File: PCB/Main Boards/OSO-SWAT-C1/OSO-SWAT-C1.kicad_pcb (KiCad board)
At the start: 4 copper layers, 24.4 x 24.4 mm, 36 parts, among them J1 OSO_SWD, J2 FH19C-9S-0.5SH_10_, Q1 Q_Photo_NPN, Q2 Q_NMOS_GSD, U1 ATSAML22J18A-MUT, U2 MIC5365-3.3YC5-TR, X1 Crystal

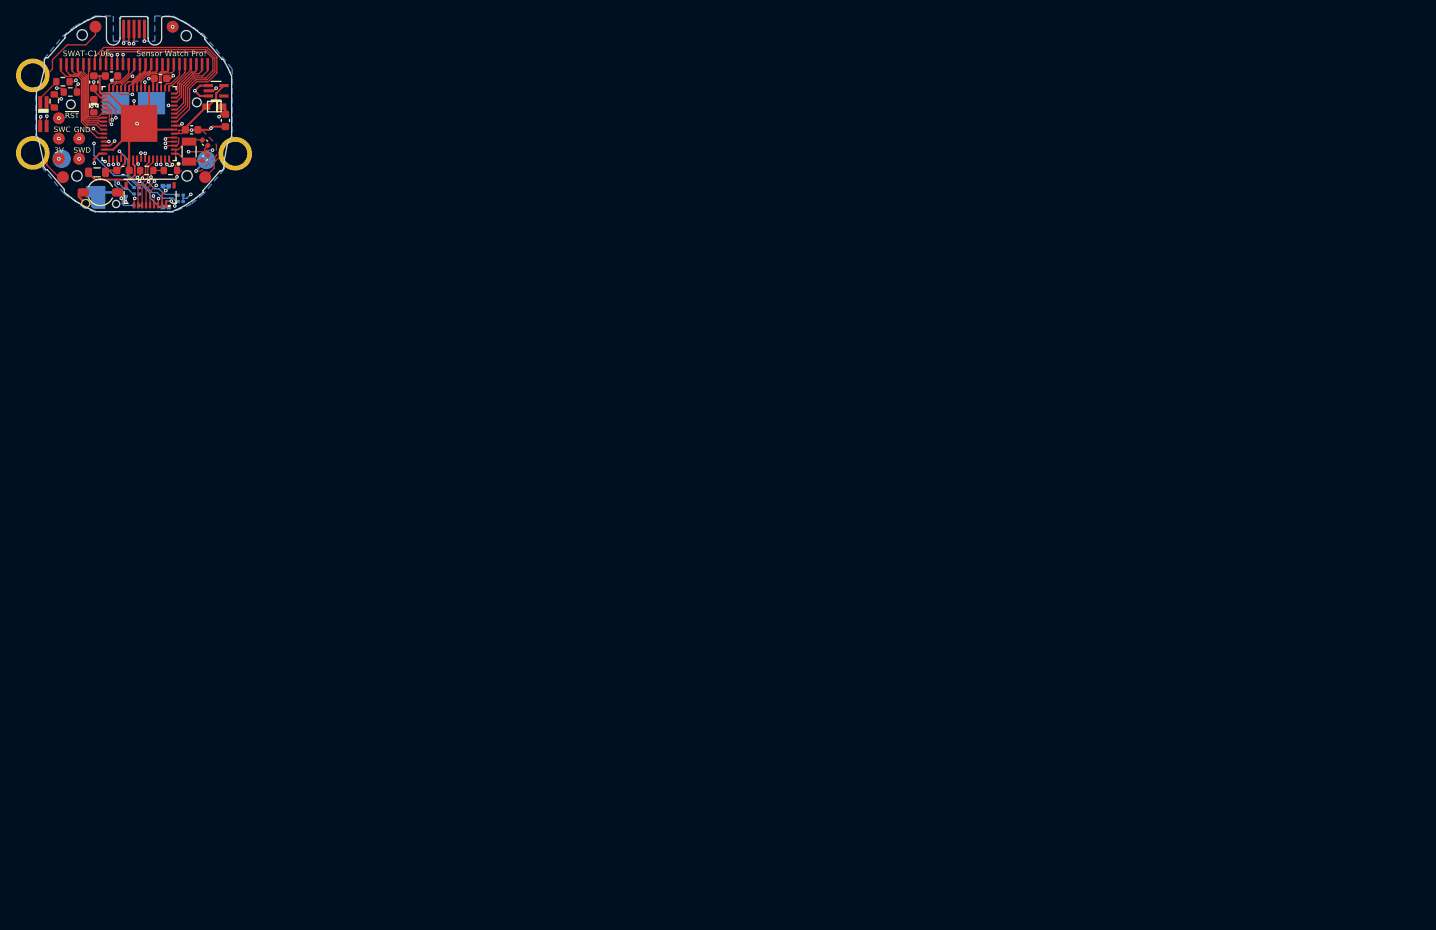
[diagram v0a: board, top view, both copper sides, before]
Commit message: Initial commit.
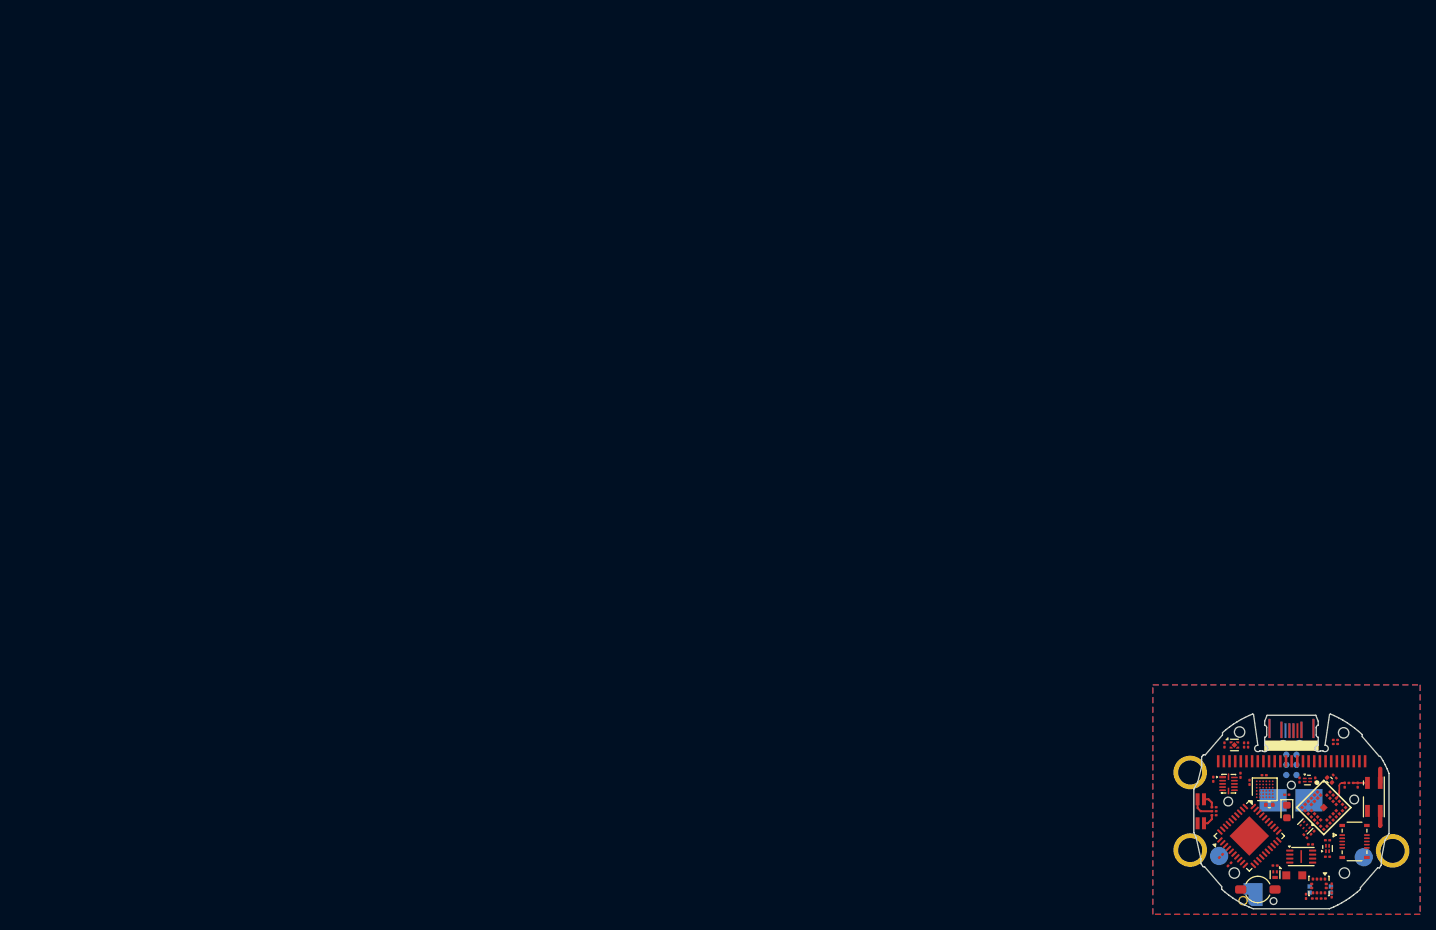
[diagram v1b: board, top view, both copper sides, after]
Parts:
- removed D1: SCHOTTKY, OSO-SWAT-A1-05:SOD-323F
- removed G***: LOGO, LOGO
- removed J1: OSO_SWD, OSO-SWD:OSO_SWD_2x3
- removed J2: FH19C-9S-0.5SH_10_, OSO-SWAT-A1-05:FH19C9S05SH10
- removed R11: 10K 0.1%, Resistor_SMD:R_0603_1608Metric
- removed R2: 10K, Resistor_SMD:R_0201_0603Metric
- removed TP10, TP8, TP9: MICROBUILDER_TESTPOINTROUND1.5MM, OSO-SWAT-A1-05:MICROBUILDER_TESTPOINT_ROUND_1.5MM
- removed X1: Crystal, Crystal:Crystal_SMD_3215-2Pin_3.2x1.5mm
- added AE1: amemb-2450AT42E0100, amemb-RF_Antenna.pretty:amemb-2450AT42E0100, F.Cu at (167.2, 97.6)
- added C10: 1uF, passives:C_0201_0603Metric_L, F.Cu at (148.0, 105.0)
- added C11: 1uF, passives:C_0201_0603Metric_L, F.Cu at (149.1, 106.0)
- added C12: 1uF, passives:C_0201_0603Metric_L, F.Cu at (159.2, 103.5)
- added C13: 1uF, passives:C_0201_0603Metric_L, F.Cu at (161.4, 103.0)
- added C14: 1uF, passives:C_0201_0603Metric_L, F.Cu at (161.4, 105.0)
- added C15: 10uF, passives:C_0402_1005Metric_L, F.Cu at (154.1, 98.6)
- added C16: 1uF, passives:C_0201_0603Metric_L, F.Cu at (151.6, 95.8)
- added C17: 1uF, passives:C_0201_0603Metric_L, F.Cu at (153.4, 94.9)
- added C46: 1uF, passives:C_0201_0603Metric_L, F.Cu at (157.9, 95.5)
- added C47: 1uF, passives:C_0201_0603Metric_L, F.Cu at (159.8, 95.5)
- added C48: 1uF, passives:C_0201_0603Metric_L, F.Cu at (150.5, 94.9)
- added C49: 1uF, passives:C_0201_0603Metric_L, F.Cu at (147.1, 95.4)
- added C50: 1uF, passives:C_0201_0603Metric_L, F.Cu at (159.5, 102.0)
- added C51: 1uF, passives:C_0201_0603Metric_L, F.Cu at (158.6, 102.5)
- added J3: Conn_ARM_SWD_TagConnect_TC2030-NL, Connector:Tag-Connect_TC2030-IDC-NL_2x03_P1.27mm_Vertical, B.Cu at (156.8, 93.6)
- added J4: Conn_02x05_Odd_Even_MountingPin, Connector_Hirose_DF40:Hirose_DF40B-10DS-0.4V_2x05-1MP_P0.4mm, F.Cu at (164.7, 103.1)
- added R5: 1kR, passives:R_0201_0603Metric_L, F.Cu at (147.2, 98.9)
- added R9: 100kR, passives:R_0201_0603Metric_L, F.Cu at (154.8, 106.2)
- added TH1: 100kR, passives:R_0201_0603Metric_L, F.Cu at (158.7, 110.0)
- added TP2: TestPoint, amemb-TestPoint.pretty:TestPoint_Pad_1.0x1.0mm_No_Silk, F.Cu at (158.2, 107.4)
- added U10: TPS22991, amemb-easyeda.pretty:4-UQFN-0.9x0.8mm, F.Cu at (158.9, 95.5)
- added U3: HJ-N54L_SIP, easyeda2kicad:COMM-SMD_L4.5-W4.5-P0.55-S0.55-TR, F.Cu at (160.9, 98.9)
- added U4: BU97930MUV-E2, Package_DFN_QFN:VQFN-40-1EP_6x6mm_P0.5mm_EP3.5x3.5mm, F.Cu at (151.6, 102.5)
- added U5: W25Q128JVE, Package_SON:Winbond_USON-8-1EP_3x2mm_P0.5mm_EP0.2x1.6mm, F.Cu at (158.1, 105.0)
- added U6: TPS22991, amemb-Package_DFN_QFN.pretty:4-UQFN-0.9x0.8mm, F.Cu at (161.4, 104.0)
- added U7: STM32L052T8Yx, Package_CSP:ST_WLCSP-36_Die417, F.Cu at (153.5, 96.6)
- added U8: TXU0204RUTR, amemb-Package_DFN_QFN.pretty:UQFN-12_L2.0-W1.7-P0.40-TL, F.Cu at (149.0, 95.9)
- added U9: TXU0101DRYR, amemb-Package_SON.pretty:SON-6_L1.5-W1.0-P0.50-TL, F.Cu at (158.6, 101.3)
- BZ1: renamed from L2; value 14 mH -> Buzzer
- C1: value 10uF -> TBD; footprint Capacitor_SMD:C_0603_1608Metric -> passives:C_0201_0603Metric_L
- C2: value 0.1uF -> TBD; footprint Capacitor_SMD:C_0201_0603Metric -> passives:C_0201_0603Metric_L; moved to F.Cu
- C3: value 0.1uF -> 220nF; footprint Capacitor_SMD:C_0603_1608Metric -> passives:C_0201_0603Metric_L
- C4: value 0.1uF -> 1uF; footprint Capacitor_SMD:C_0603_1608Metric -> passives:C_0201_0603Metric_L
- C5, C9: footprint Capacitor_SMD:C_0603_1608Metric -> passives:C_0201_0603Metric_L
- C6: value 1uF -> 10uF; footprint Capacitor_SMD:C_0603_1608Metric -> passives:C_0402_1005Metric_L
- C7, C8: value 22pf -> 1uF; footprint Capacitor_SMD:C_0402_1005Metric -> passives:C_0201_0603Metric_L
- L1: value 10uH -> 0R; footprint Inductor_SMD:L_0805_2012Metric -> passives:R_0201_0603Metric_L
- Q1: footprint Resistor_SMD:R_0603_1608Metric -> Diode_SMD:D_0603_1608Metric
- Q2: footprint Package_TO_SOT_SMD:SOT-523 -> Package_DFN_QFN:Diodes_DFN1006-3; moved to F.Cu
- R1: value 10K -> 10kR; footprint Resistor_SMD:R_0201_0603Metric -> passives:R_0201_0603Metric_L; moved to F.Cu
- R10: value 10K THERM -> 100kR; footprint Resistor_SMD:R_0603_1608Metric -> passives:R_0201_0603Metric_L
- R3: value 10K -> 100kR, 0.1%; footprint Resistor_SMD:R_0201_0603Metric -> passives:R_0201_0603Metric_L; moved to F.Cu
- R4: value 10K -> 100R; footprint Resistor_SMD:R_0201_0603Metric -> passives:R_0201_0603Metric_L; moved to F.Cu
- R6: value 1K -> 100R; footprint Resistor_SMD:R_0603_1608Metric -> passives:R_0201_0603Metric_L
- R7, R8: value 100 -> 5.1kR; footprint Resistor_SMD:R_0603_1608Metric -> passives:R_0201_0603Metric_L
- TP1: value MICROBUILDER_TESTPOINTROUND1.5MM -> TestPoint; footprint OSO-SWAT-A1-05:MICROBUILDER_TESTPOINT_ROUND_1.5MM -> amemb-TestPoint.pretty:TestPoint_Pad_1.0x1.0mm_No_Silk
- U1: value ATSAML22J18A-MUT -> NCP115AMX250TCG; footprint OSO-SWAT-A1-05:QFN64_9X9MC_MCH -> Package_DFN_QFN:OnSemi_XDFN4-1EP_1.0x1.0mm_EP0.52x0.52mm
- U2: value MIC5365-3.3YC5-TR -> ADXL367; footprint OSO-SWAT-A1-05:SOT65P210X110-5N -> amemb-Package_LGA.pretty:amemb-ADXL367_LGA-12_2.11x2.21mm_P0.5mm_LayoutBorder2x4y
- moved C3 184.5 mm to (160.8, 110.3), turned to 0 degrees
- moved R7 179.3 mm to (162.4, 91.0)
- moved C4 177.8 mm to (161.9, 108.7), turned to -90 degrees
- moved R8 177.7 mm to (162.4, 90.5)
- moved C5 176.2 mm to (161.9, 109.8), turned to -90 degrees
- moved C6 175.9 mm to (161.6, 95.5), turned to 135 degrees
- moved TP1 175.0 mm to (156.2, 107.4)
- moved L1 174.3 mm to (164.3, 95.8), turned to 0 degrees
- moved Q1 173.3 mm to (156.3, 99.4)
- moved R6 170.0 mm to (147.2, 99.4), turned to 0 degrees
- moved U2 170.0 mm to (160.3, 108.7), turned to -90 degrees
- moved C2 169.0 mm to (165.1, 96.1), turned to -90 degrees
- moved BZ1 168.9 mm to (152.7, 109.1)
- moved U$2 168.9 mm to (156.8, 99.4)
- moved D2 168.9 mm to (145.5, 99.4)
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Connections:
- BZ1 pad 1: /BUZZER_HV -> VDD
- BZ1 pad 2: VCC -> /BUZZER_HV
- C1 pad 1: VCC -> Net-(U3-RF)
- C2 pad 1: VCC -> Net-(AE1-FEED)
- C3 pad 1: VCC -> Net-(U2-V_{REG_OUT})
- C4 pad 1: VCC -> VDD
- C5 pad 1: /VDDCORE -> VDD
- C6 pad 1: /VLCD -> VDD
- C7 pad 1: /XIN32 -> VDD
- C8 pad 1: /XOUT32 -> VBUS
- C9 pad 1: +3V3 -> Net-(U1-OUT)
- D2 pad 2: VCC -> VDD
- L1 pad 1: /VDDCORE -> Net-(U3-RF)
- L1 pad 2: /VDDOUT -> Net-(AE1-FEED)
- R1 pad 1: VCC -> VDD
- R10 pad 1: VCC -> VBUS
- R10 pad 2: /TEMPSENSE -> GND
- R3 pad 1: VCC -> /TEMPSENSE
- R3 pad 2: /SCL -> /~{TS_ENABLE}
- R4 pad 1: VCC -> Net-(D2C-CB)
- R4 pad 2: /SDA -> /~{BLUE}
- R6 pad 1: /~{GREEN} -> Net-(D2A-CR)
- R6 pad 2: Net-(D2B-CG) -> /~{RED}
- R7 pad 1: /~{RED} -> GND
- R7 pad 2: Net-(D2A-CR) -> Net-(R7-Pad2)
- R8 pad 1: /~{BLUE} -> GND
- R8 pad 2: Net-(D2C-CB) -> Net-(R8-Pad2)
- U$2 pad LIGHT: /SWCLK_LIGHT -> /LIGHT
- U$2 pad MODE: /SWDIO_MODE -> /MODE
- U$2 pad VCC1: VCC -> VDD
- U$2 pad VCC2: VCC -> VDD
- U1 pad 1: /XIN32 -> Net-(U1-OUT)
- U1 pad 2: /XOUT32 -> GND
- U1 pad 3: /ALARM -> VBUS
- U1 pad 4: /TEMPSENSE -> VBUS
- U1 pad 5: /A0 -> GND
- U2 pad 1: VBUS -> unconnected-(U2-SCLK-Pad1)
- U2 pad 2: GND -> unconnected-(U2-MOSI-Pad2)
- U2 pad 3: VBUS -> unconnected-(U2-MISO-Pad3)
- U2 pad 4: (no net) -> unconnected-(U2-~{CS}-Pad4)
- U2 pad 5: +3V3 -> unconnected-(U2-INT1-Pad5)
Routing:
- net GND: track 58.7 -> 3.63 mm, vias 14 -> 0
- net /SWCLK_LIGHT: track 32.1 -> 0.00 mm, vias 2 -> 0
- net /COM0: track 28.5 -> 0.00 mm
- net VCC: track 26.7 -> 0.00 mm, vias 13 -> 0
- net /COM1: track 26.6 -> 0.00 mm
- net /LIGHTSENSE: track 24.8 -> 0.00 mm, vias 3 -> 0
- net /COM2: track 24.8 -> 0.00 mm
- net /~{RESET}: track 21.9 -> 0.00 mm, vias 2 -> 0
- net /SWDIO_MODE: track 18.8 -> 0.00 mm, vias 2 -> 0
- net VBUS: track 17.6 -> 0.00 mm, vias 2 -> 0
- net /USB_P: track 16.6 -> 0.00 mm, vias 2 -> 0
- net /USB_N: track 15.9 -> 0.00 mm, vias 2 -> 0
- net /VLCD: track 14.3 -> 0.00 mm, vias 3 -> 0
- net /SEG15: track 13.5 -> 0.00 mm, vias 2 -> 0
- net /SCL: track 13.3 -> 0.00 mm, vias 1 -> 0
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- added copper zone on In1.Cu, net GND
- removed copper zone on In1.Cu, net VCC
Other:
- board size 24.4 x 24.4 mm -> 24.4 x 24.3 mm
- board text removed: "3V"
- board text removed: "9-Pin connector:"
- board text removed: "A0: PB04 SDA: PB30/SERCOM1.0 SCL: PB31/SERCOM1.1 A1/SCK:PB01/TC3.1/S3.3 A2/MOSI:PB02/TC2.0/S3.0 A3/CS: PB03/TC2.1 A4/MISO: PB00/TC3.0 /S3.2"
- board text removed: "Alarm btn: PA02/ I2/ RTC. IN2"
- board text removed: "CC-BY-SA 4.0"
- board text removed: "GND"
- board text removed: "IMPORTANT:"
- board text removed: "Light + Sound: ~Red: PA12/TCC.6 ~Blue: PA13/TCC.7 ~Green: PA22/TCC.4 Piezo: PA27/TCC.5"
- board text removed: "Light Btn: PA30/I10 Temp Sense: PA03 TS ~Enable: PB23 Light Sense: PA04 LS ~Enable: PB22"
- board text removed: "Mode Btn: PA31/I11"
- board text removed: "REMOVE BAT B4 USING USB!!!"
- board text removed: "RESET"
- board text removed: "SWAT-C1-06"
- board text removed: "SWC"
- board text removed: "SWD"
- board text removed: "Sensor Watch Pro!"
- board text removed: "by joey castillo"
- board text removed: "~{RST}"
